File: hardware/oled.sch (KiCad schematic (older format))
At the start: 4 parts

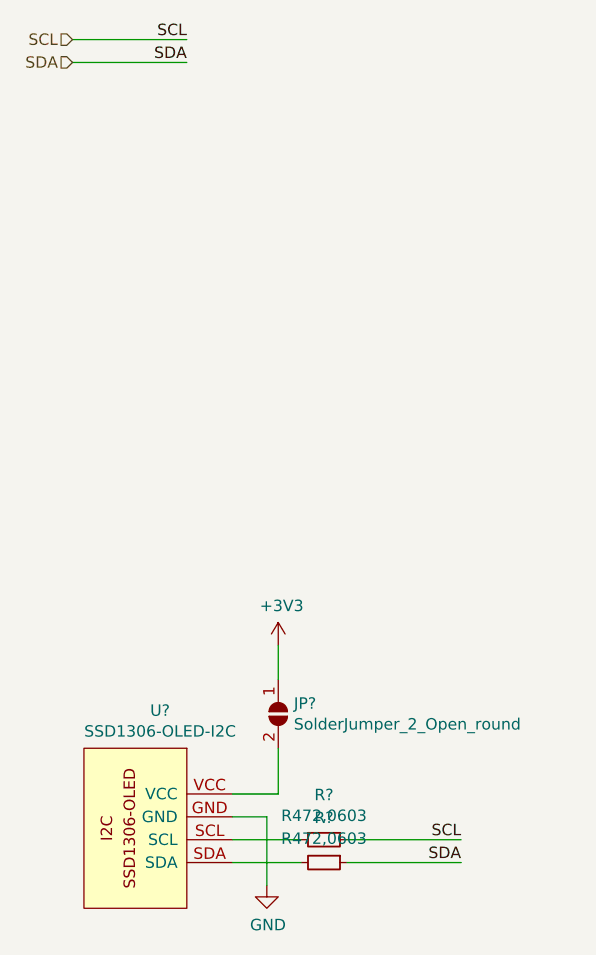
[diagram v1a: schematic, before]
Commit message: update for power symbol,
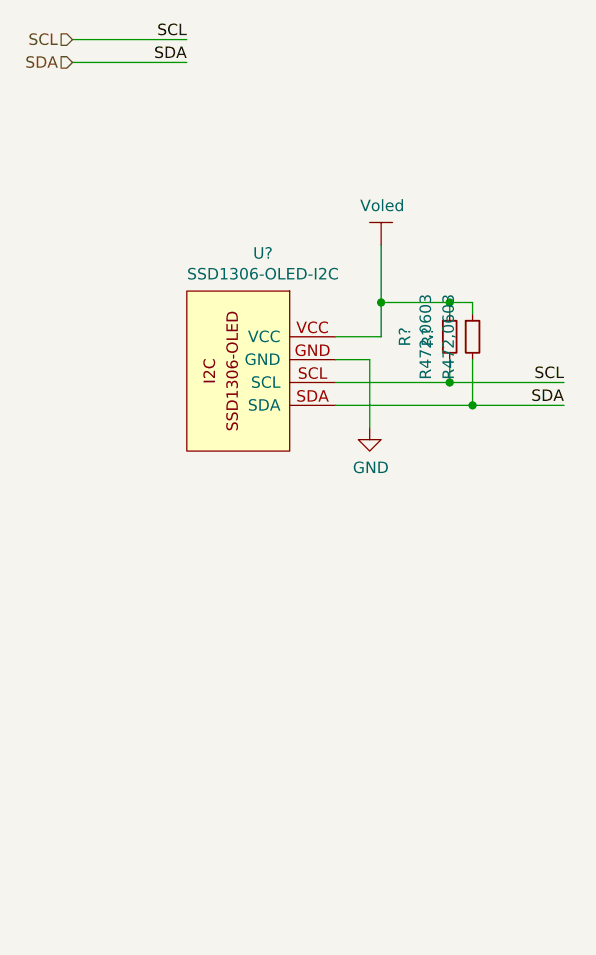
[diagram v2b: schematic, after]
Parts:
- removed JP?: SolderJumper_2_Open_round, Jumper:SolderJumper-2_P1.3mm_Open_RoundedPad1.0x1.5mm, symbol my_solder_jumper:SolderJumper_2_Open_round
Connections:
- net SCL: now also R?.2, U?.SCL; no longer R?.1
- net SDA: now also R?.2, U?.SDA; no longer R?.1
- net Voled: now reaches U?.VCC
- net Voled: now also R?.1, R?.1
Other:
- moved on the sheet: R?, U?
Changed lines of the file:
@@
 L taobao-board:SSD1306-OLED-I2C U?
 U 1 1 5D09D217
-P 1600 4250
-F 0 "U?" H 1717 4765 50  0000 C CNN
-F 1 "SSD1306-OLED-I2C" H 1717 4674 50  0000 C CNN
-F 2 "" H 1600 4100 50  0001 C CNN
-F 3 "" H 1600 4100 50  0001 C CNN
-	1    1600 4250
+P 2050 2250
+F 0 "U?" H 2167 2765 50  0000 C CNN
+F 1 "SSD1306-OLED-I2C" H 2167 2674 50  0000 C CNN
+F 2 "" H 2050 2100 50  0001 C CNN
+F 3 "" H 2050 2100 50  0001 C CNN
+	1    2050 2250
 	-1   0    0    -1
-$EndComp
-$Comp
-L power:+3V3 #PWR?
-U 1 1 5D09D7EA
-P 2000 3450
-F 0 "#PWR?" H 2000 3300 50  0001 C CNN
-F 1 "+3V3" H 2015 3623 50  0000 C CNN
-F 2 "" H 2000 3450 50  0001 C CNN
-F 3 "" H 2000 3450 50  0001 C CNN
-	1    2000 3450
-	1    0    0    -1
-$EndComp
-$Comp
-L my_solder_jumper:SolderJumper_2_Open_round JP?
-U 1 1 5D09E183
-P 2000 3750
-F 0 "JP?" V 1954 3818 50  0000 L CNN
-F 1 "SolderJumper_2_Open_round" V 2045 3818 50  0000 L CNN
-F 2 "Jumper:SolderJumper-2_P1.3mm_Open_RoundedPad1.0x1.5mm" H 2000 3750 50  0001 C CNN
-F 3 "~" H 2000 3750 50  0001 C CNN
-	1    2000 3750
-	0    1    1    0
 $EndComp
 $Comp
 L power:GND #PWR?
 U 1 1 5D09E684
-P 1950 4500
-F 0 "#PWR?" H 1950 4250 50  0001 C CNN
-F 1 "GND" H 1955 4327 50  0000 C CNN
-F 2 "" H 1950 4500 50  0001 C CNN
-F 3 "" H 1950 4500 50  0001 C CNN
-	1    1950 4500
+P 2400 2500
+F 0 "#PWR?" H 2400 2250 50  0001 C CNN
+F 1 "GND" H 2405 2327 50  0000 C CNN
+F 2 "" H 2400 2500 50  0001 C CNN
+F 3 "" H 2400 2500 50  0001 C CNN
+	1    2400 2500
 	1    0    0    -1
 $EndComp
@@
 L taobao-r:R472,0603 R?
 U 1 1 5D09E950
-P 2200 4300
-F 0 "R?" V 2004 4300 50  0000 C CNN
-F 1 "R472,0603" V 2095 4300 50  0000 C CNN
-F 2 "Resistor_SMD:R_0603_1608Metric_Pad1.05x0.95mm_HandSolder" H 2200 4300 50  0001 C CNN
-F 3 "~" H 2200 4300 50  0001 C CNN
-	1    2200 4300
-	0    1    1    0
+P 2750 2100
+F 0 "R?" V 2554 2100 50  0000 C CNN
+F 1 "R472,0603" V 2645 2100 50  0000 C CNN
+F 2 "Resistor_SMD:R_0603_1608Metric_Pad1.05x0.95mm_HandSolder" H 2750 2100 50  0001 C CNN
+F 3 "~" H 2750 2100 50  0001 C CNN
+	1    2750 2100
+	1    0    0    -1
 $EndComp
 $Comp
 L taobao-r:R472,0603 R?
 U 1 1 5D09EC8C
-P 2200 4400
-F 0 "R?" V 2004 4400 50  0000 C CNN
-F 1 "R472,0603" V 2095 4400 50  0000 C CNN
-F 2 "Resistor_SMD:R_0603_1608Metric_Pad1.05x0.95mm_HandSolder" H 2200 4400 50  0001 C CNN
-F 3 "~" H 2200 4400 50  0001 C CNN
-	1    2200 4400
-	0    1    1    0
+P 2850 2100
+F 0 "R?" V 2654 2100 50  0000 C CNN
+F 1 "R472,0603" V 2745 2100 50  0000 C CNN
+F 2 "Resistor_SMD:R_0603_1608Metric_Pad1.05x0.95mm_HandSolder" H 2850 2100 50  0001 C CNN
+F 3 "~" H 2850 2100 50  0001 C CNN
+	1    2850 2100
+	1    0    0    -1
 $EndComp
-Wire Wire Line
-	1800 4300 2100 4300
-Wire Wire Line
-	1800 4400 2100 4400
-Text Label 2800 4400 2    50   ~ 0
+Text Label 3250 2400 2    50   ~ 0
 SDA
-Text Label 2800 4300 2    50   ~ 0
+Text Label 3250 2300 2    50   ~ 0
 SCL
 Wire Wire Line
-	2300 4300 2800 4300
+	2400 2500 2400 2200
 Wire Wire Line
-	2800 4400 2300 4400
+	2400 2200 2250 2200
 Wire Wire Line
-	1950 4500 1950 4200
+	2250 2100 2450 2100
 Wire Wire Line
-	1950 4200 1800 4200
-Wire Wire Line
-	1800 4100 2000 4100
-Wire Wire Line
-	2000 4100 2000 3900
-Wire Wire Line
-	2000 3450 2000 3600
+	2450 2100 2450 1950
 Text Label 1600 900  2    50   ~ 0
 SDA
@@
 Text HLabel 1100 800  0    50   Input ~ 0
 SCL
+Wire Wire Line
+	2250 2300 2750 2300
+Wire Wire Line
+	2250 2400 2850 2400
+Wire Wire Line
+	2450 1950 2750 1950
+Wire Wire Line
+	2750 1950 2750 2000
+Connection ~ 2450 1950
+Wire Wire Line
+	2750 1950 2850 1950
+Wire Wire Line
+	2850 1950 2850 2000
+Connection ~ 2750 1950
+Wire Wire Line
+	2750 2200 2750 2300
+Connection ~ 2750 2300
+Wire Wire Line
+	2750 2300 3250 2300
+Wire Wire Line
+	2850 2200 2850 2400
+Connection ~ 2850 2400
+Wire Wire Line
+	2850 2400 3250 2400
+$Comp
+L my_power:Voled #PWR?
+U 1 1 5D0FFF44
+P 2450 1700
+F 0 "#PWR?" H 2450 1550 50  0001 C CNN
+F 1 "Voled" H 2455 1873 50  0000 C CNN
+F 2 "" H 2450 1700 50  0001 C CNN
+F 3 "" H 2450 1700 50  0001 C CNN
+	1    2450 1700
+	1    0    0    -1
+$EndComp
+Wire Wire Line
+	2450 1700 2450 1950
 $EndSCHEMATC

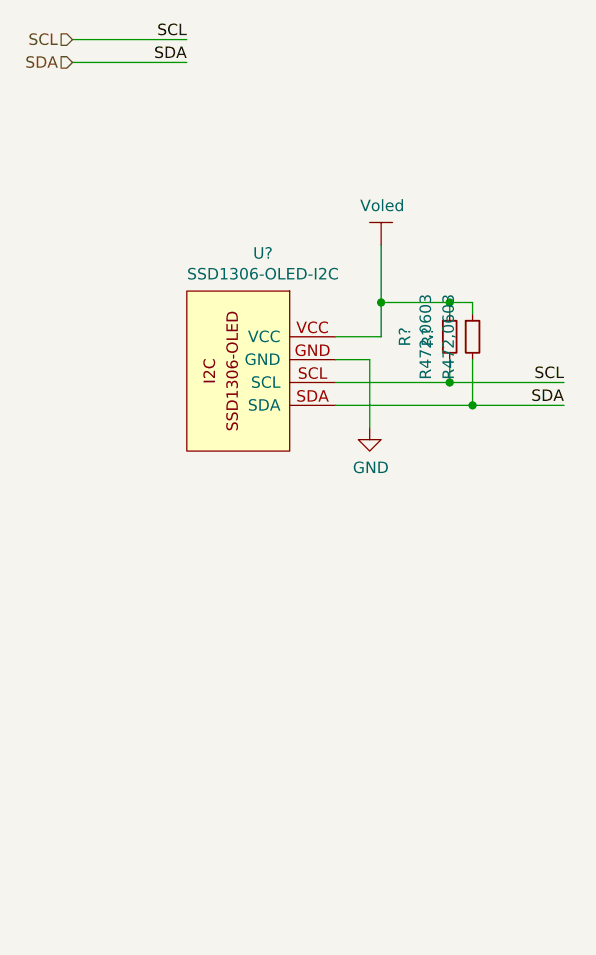
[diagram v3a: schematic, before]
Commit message: update,
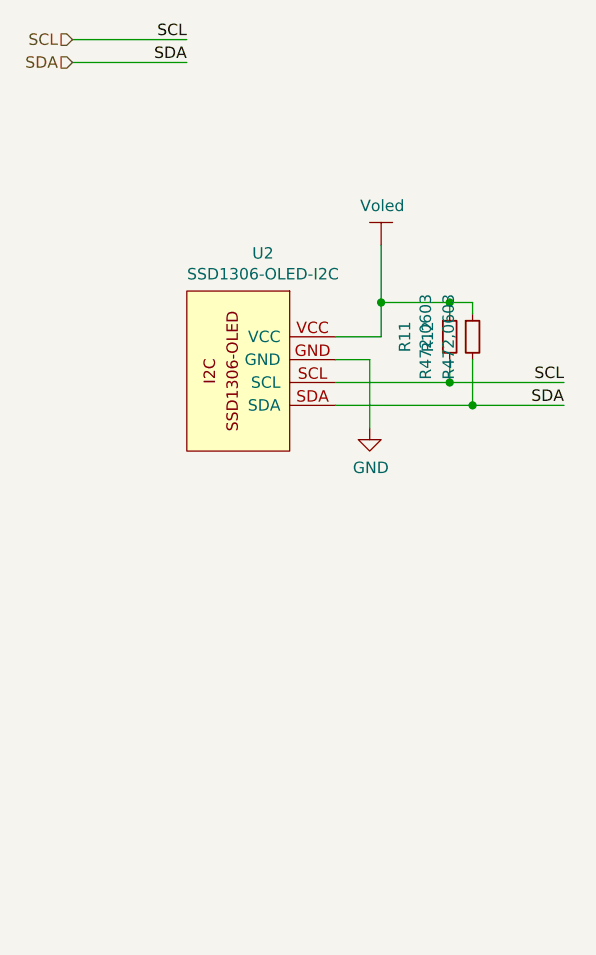
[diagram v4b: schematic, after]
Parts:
- gave numbers to parts that had none: 3
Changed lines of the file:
@@
 $EndBitmap
 $Comp
-L taobao-board:SSD1306-OLED-I2C U?
+L taobao-board:SSD1306-OLED-I2C U2
 U 1 1 5D09D217
 P 2050 2250
-F 0 "U?" H 2167 2765 50  0000 C CNN
+F 0 "U2" H 2167 2765 50  0000 C CNN
 F 1 "SSD1306-OLED-I2C" H 2167 2674 50  0000 C CNN
 F 2 "" H 2050 2100 50  0001 C CNN
@@
 $EndComp
 $Comp
-L power:GND #PWR?
+L power:GND #PWR019
 U 1 1 5D09E684
 P 2400 2500
-F 0 "#PWR?" H 2400 2250 50  0001 C CNN
+F 0 "#PWR019" H 2400 2250 50  0001 C CNN
 F 1 "GND" H 2405 2327 50  0000 C CNN
 F 2 "" H 2400 2500 50  0001 C CNN
@@
 $EndComp
 $Comp
-L taobao-r:R472,0603 R?
+L taobao-r:R472,0603 R11
 U 1 1 5D09E950
 P 2750 2100
-F 0 "R?" V 2554 2100 50  0000 C CNN
+F 0 "R11" V 2554 2100 50  0000 C CNN
 F 1 "R472,0603" V 2645 2100 50  0000 C CNN
 F 2 "Resistor_SMD:R_0603_1608Metric_Pad1.05x0.95mm_HandSolder" H 2750 2100 50  0001 C CNN
@@
 $EndComp
 $Comp
-L taobao-r:R472,0603 R?
+L taobao-r:R472,0603 R12
 U 1 1 5D09EC8C
 P 2850 2100
-F 0 "R?" V 2654 2100 50  0000 C CNN
+F 0 "R12" V 2654 2100 50  0000 C CNN
 F 1 "R472,0603" V 2745 2100 50  0000 C CNN
 F 2 "Resistor_SMD:R_0603_1608Metric_Pad1.05x0.95mm_HandSolder" H 2850 2100 50  0001 C CNN
@@
 	2850 2400 3250 2400
 $Comp
-L my_power:Voled #PWR?
+L my_power:Voled #PWR018
 U 1 1 5D0FFF44
 P 2450 1700
-F 0 "#PWR?" H 2450 1550 50  0001 C CNN
+F 0 "#PWR018" H 2450 1550 50  0001 C CNN
 F 1 "Voled" H 2455 1873 50  0000 C CNN
 F 2 "" H 2450 1700 50  0001 C CNN
